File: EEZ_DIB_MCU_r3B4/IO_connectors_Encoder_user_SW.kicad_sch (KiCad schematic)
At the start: 36 parts, among them IC1 TPD4E001DRLR, IC2 74AUP1G74DC.125, IC3 CD74HC4050PWR, SW1 TL1100CF160Q, SW2 PEC16-2215F-S0024, X1 DS1024-2*20R0, X2 DS1013-16SSIB1, X3 691322110005

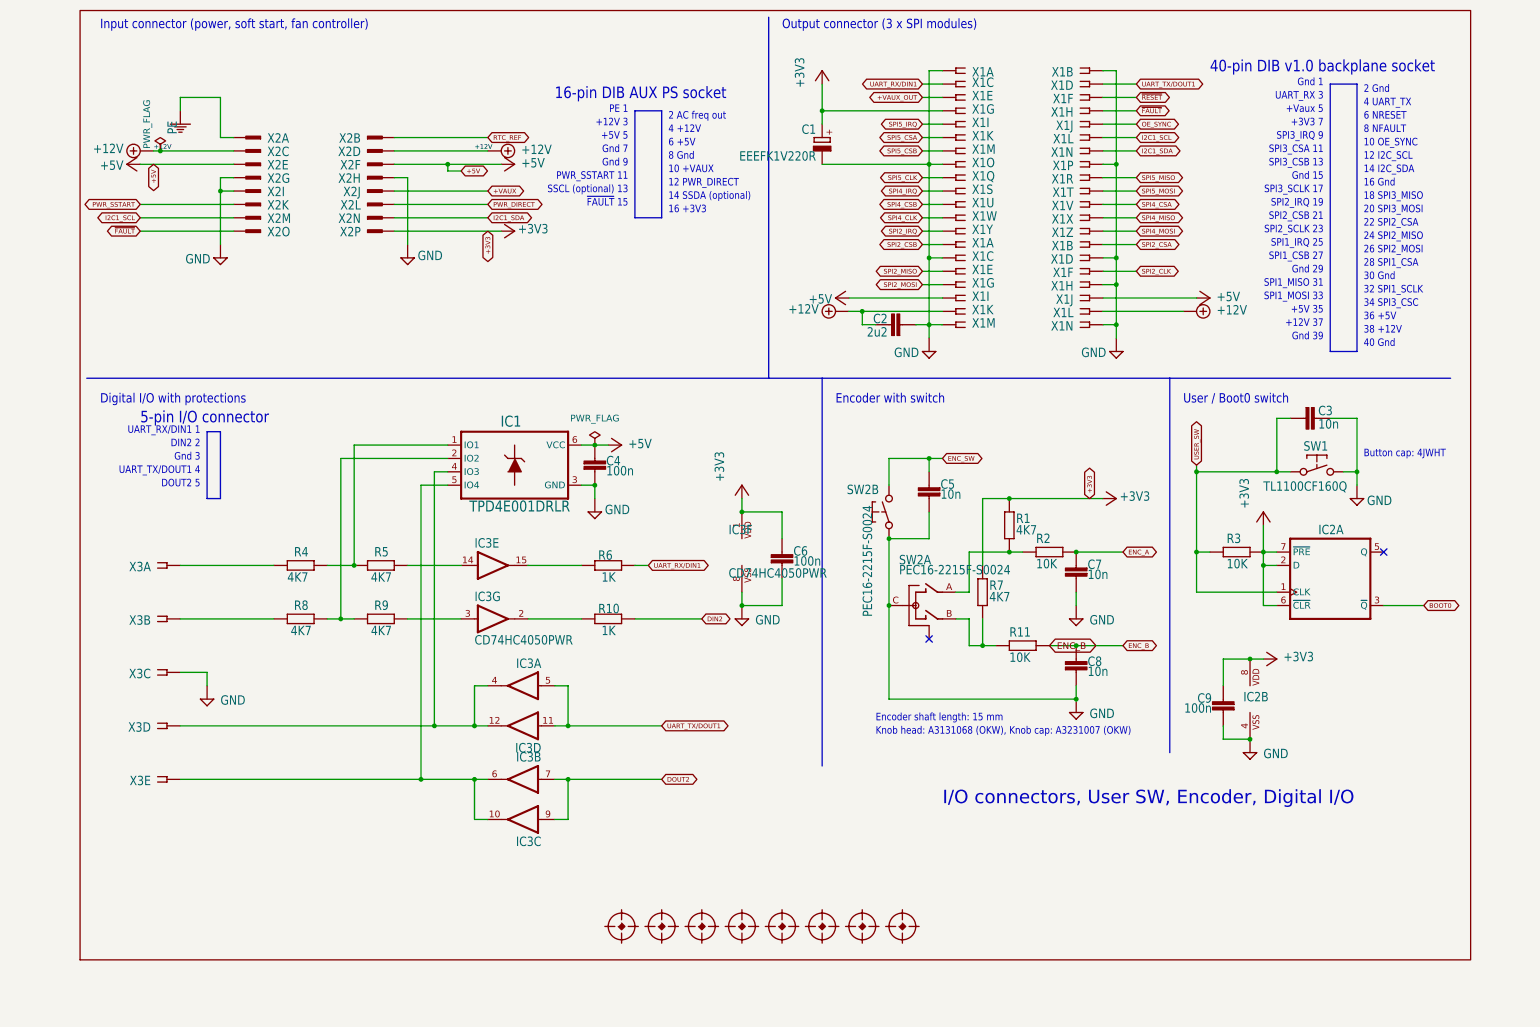
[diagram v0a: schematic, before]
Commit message: Adding temperary PCIe connector - adding logos
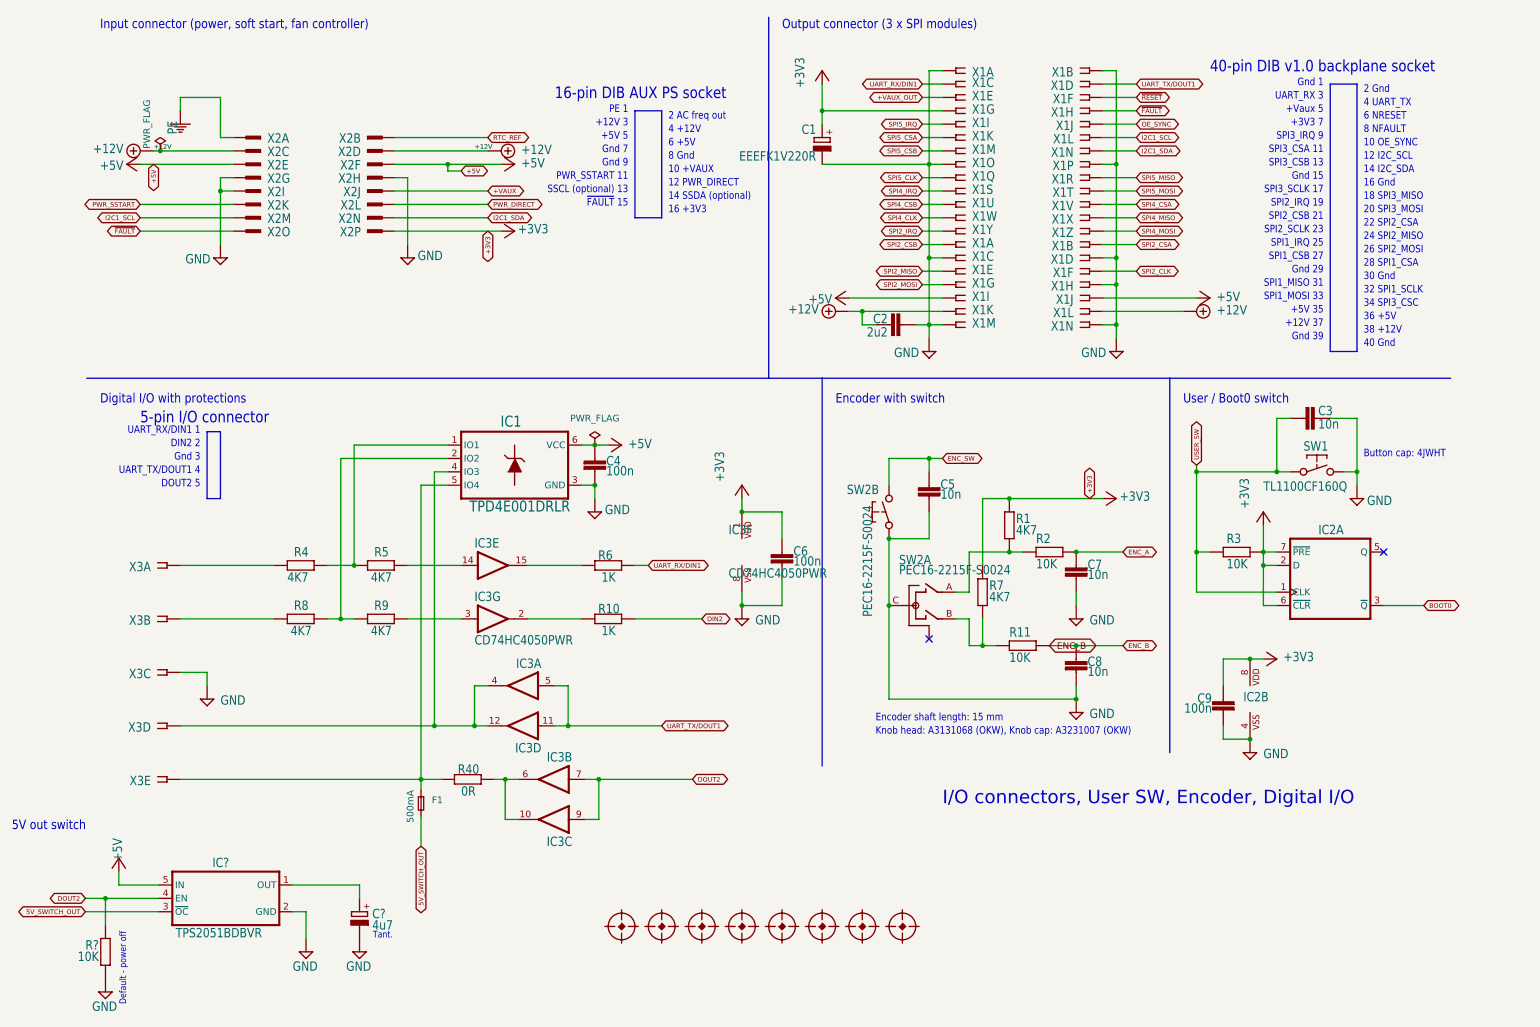
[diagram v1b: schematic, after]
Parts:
- added C?: 4u7, EEZ_DIB_MCU_r3B4:EC1206, symbol EEZ_DIB_MCU_r3B4-eagle-import:ECAP1206
- added F1: 500mA, Fuse:Fuse_0805_2012Metric, symbol Device:Fuse_Small
- added IC?: TPS2051BDBVR, EEZ_DIB_MCU_r3B4:DBV5, symbol EEZ_DIB_MCU_r3B4-eagle-import:TPS2051B
- added R40: 0R, Resistor_SMD:R_0603_1608Metric, symbol EEZ_DIB_MCU_r3B4-eagle-import:R-EU_R0805
- added R?: 10K, Resistor_SMD:R_0603_1608Metric, symbol EEZ_DIB_MCU_r3B4-eagle-import:R-EU_R0805
- C1: footprint EEZ_DIB_MCU_r3B4:PANASONIC_C -> Fuse:Fuse_0805_2012Metric
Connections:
- net +5V: now also IC?.5 (IN)
- net DOUT2: now also IC?.4 (EN), R?.2
- net GND: now also C?.-, IC?.2 (GND), R?.1
- net at IC1.5 (IO4), X3.5 (1): now also F1.1, R40.1; no longer IC3.10 (O), IC3.6 (O)
- new net: IC3.10 (O), IC3.6 (O), R40.2
- new net: C?.+, IC?.1 (OUT)
- new net 5V_SWITCH_OUT: F1.2, IC?.3 (~{OC})
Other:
- note added: "5V out switch"
- note added: "Default - power off"
- note added: "Tant."
- moved on the sheet: IC3B, IC3C
